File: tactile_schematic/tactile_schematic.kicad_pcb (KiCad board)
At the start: 2 copper layers, 89.3 x 58.4 mm, 37 parts, among them IC1 CY8C4145PVI-PS431, J1 Conn_01x02, J2 Conn_01x04, J3 Conn_01x04, J4 Conn_01x02

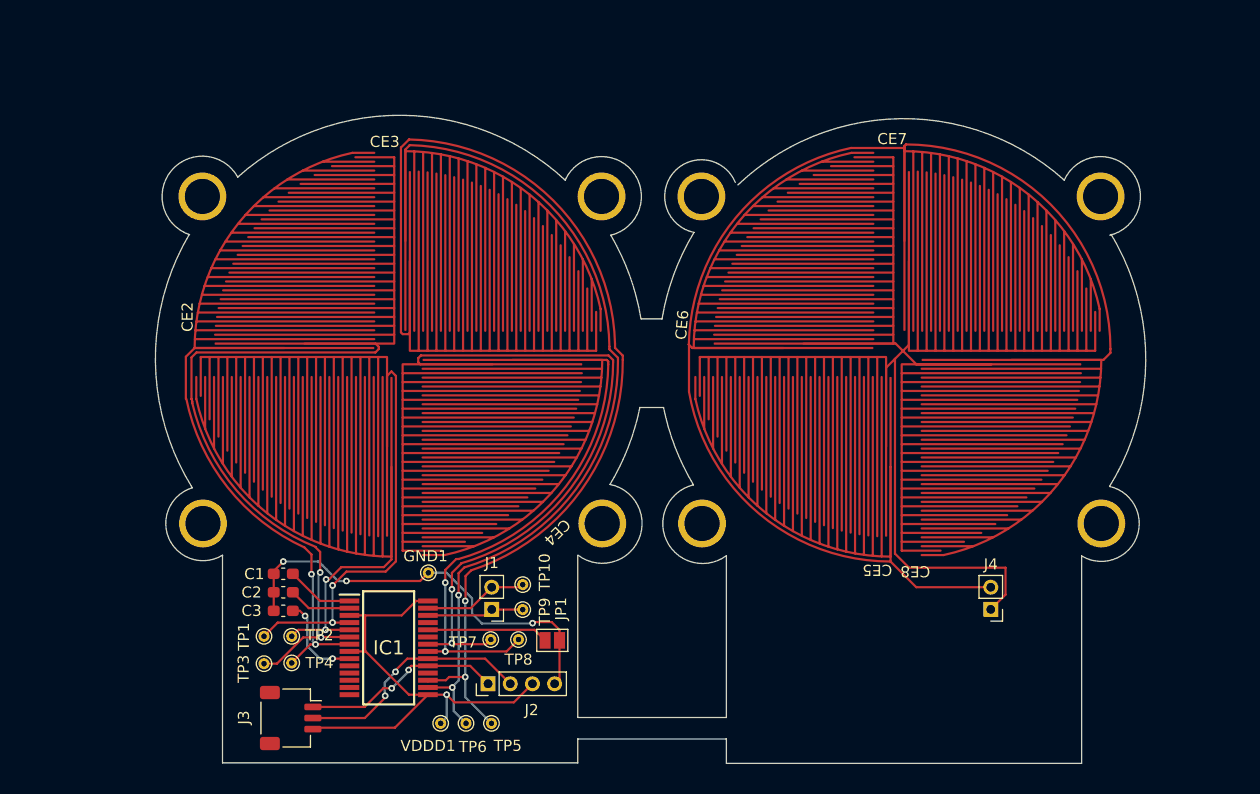
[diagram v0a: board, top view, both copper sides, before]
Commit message: PCB first draft
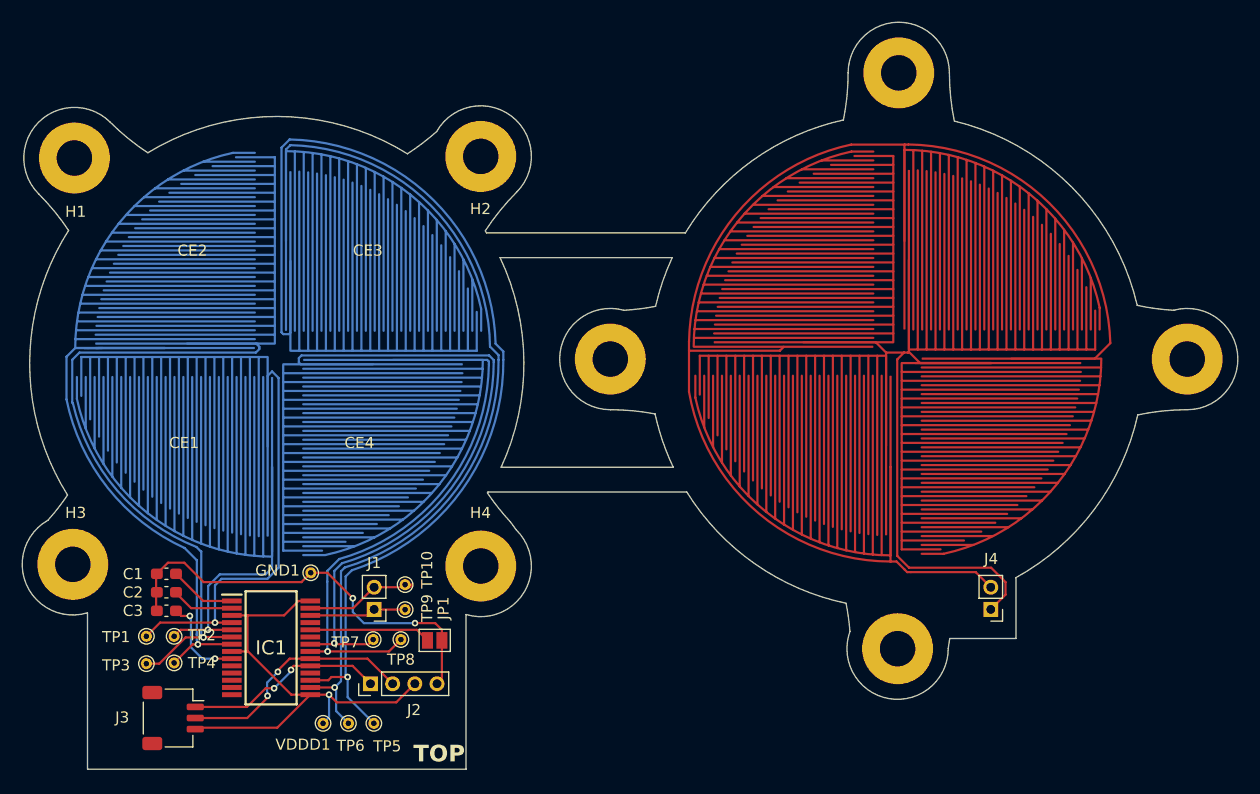
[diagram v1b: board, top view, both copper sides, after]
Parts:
- CE1, CE2, CE3, CE4: footprint PCB Coils:COIL_GENERATOR -> PCB Coils:COIL_GENERATOR_1
- H1, H2, H3, H4, H5, H6, H7, H8: footprint ECE445L:MountingHole_4_40 -> MountingHole:MountingHole_3.2mm_M3_Pad
- moved H3 47.9 mm to (168.3, 69.6)
- moved H4 25.3 mm to (205.1, 69.7)
- moved H7 21.6 mm to (242.7, 77.2)
- moved H5 21.0 mm to (242.8, 25.3)
- moved H8 17.0 mm to (216.8, 51.1)
- moved H6 16.6 mm to (268.8, 51.1)
- moved H1 12.0 mm to (168.5, 33.0)
- moved H2 11.5 mm to (205.1, 32.8)
- moved CE1 10.8 mm to (186.3, 50.9)
- moved CE2 10.8 mm to (186.6, 50.1)
- moved CE3 10.8 mm to (187.6, 50.3)
- moved CE4 10.8 mm to (187.3, 51.2)
- moved GND1 10.6 mm to (189.8, 70.4)
- moved IC1 10.6 mm to (186.2, 77.1)
- moved J1 10.6 mm to (195.5, 73.7)
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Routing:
- net P1.3: track 28.1 -> 36.0 mm, vias 2 -> 1
- net P1.1: track 25.0 -> 32.6 mm, vias 2 -> 1
- net P5.2: track 83.3 -> 82.5 mm
- net P1.0: track 42.4 -> 42.9 mm, vias 2 -> 1
- net P1.2: track 45.6 -> 45.4 mm, vias 2 -> 1
- net P0.0: track 26.8 -> 26.6 mm, vias 2 -> 1
- net GND: track 38.9 -> 38.7 mm, vias 3 -> 2
- net P3.2: track 45.4 -> 45.5 mm, vias 2 -> 1
- net P0.1: track 38.7 -> 38.6 mm, vias 2 -> 1
- net P3.1: track 27.7 -> 27.6 mm, vias 2 -> 1
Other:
- board size 89.3 x 58.4 mm -> 109.6 x 67.4 mm
- board text added: "BOTTOM"
- board text added: "H2"
- board text added: "TOP"
